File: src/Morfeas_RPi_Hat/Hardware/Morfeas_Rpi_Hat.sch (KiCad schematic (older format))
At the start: 49 parts, among them J1 Power IN, J2 RPi_header, J3 CAN0_Power+, J4 CAN1_Power+, J5 RS_232, Q1 SUM110P06, Q2 SUM110P06, U1 DS3231, U2 TSR2-2450, U3 TLV70433, U4 SP3232, U5 24AA08, U6 MAX9611, U7 MAX9611

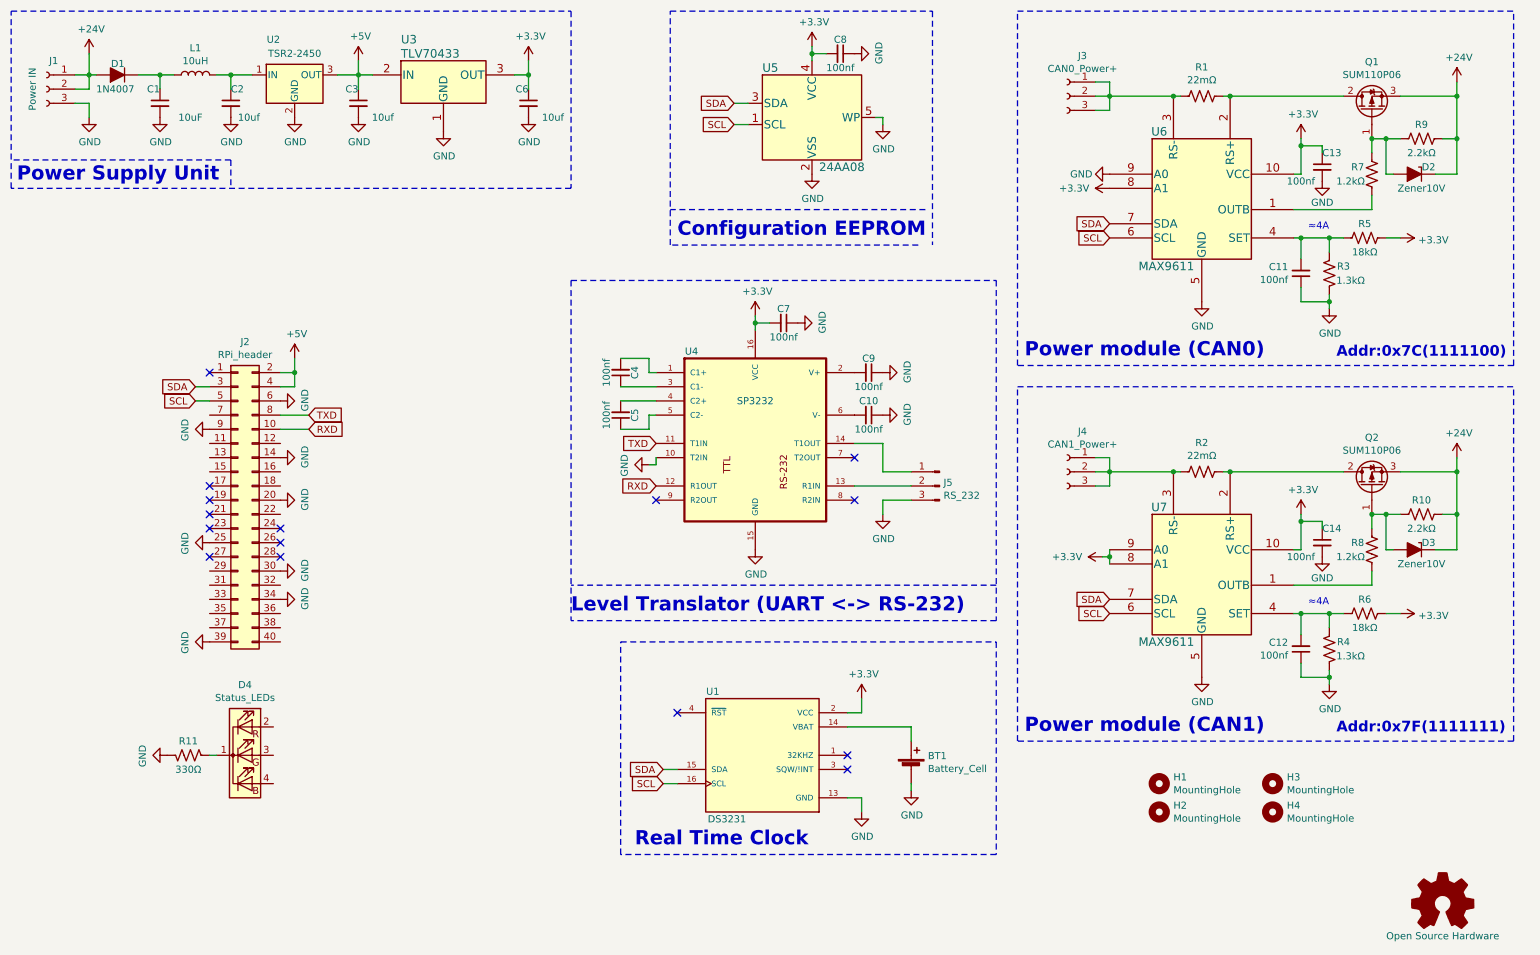
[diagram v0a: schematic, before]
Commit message: Update Morfeas_RPi_hat
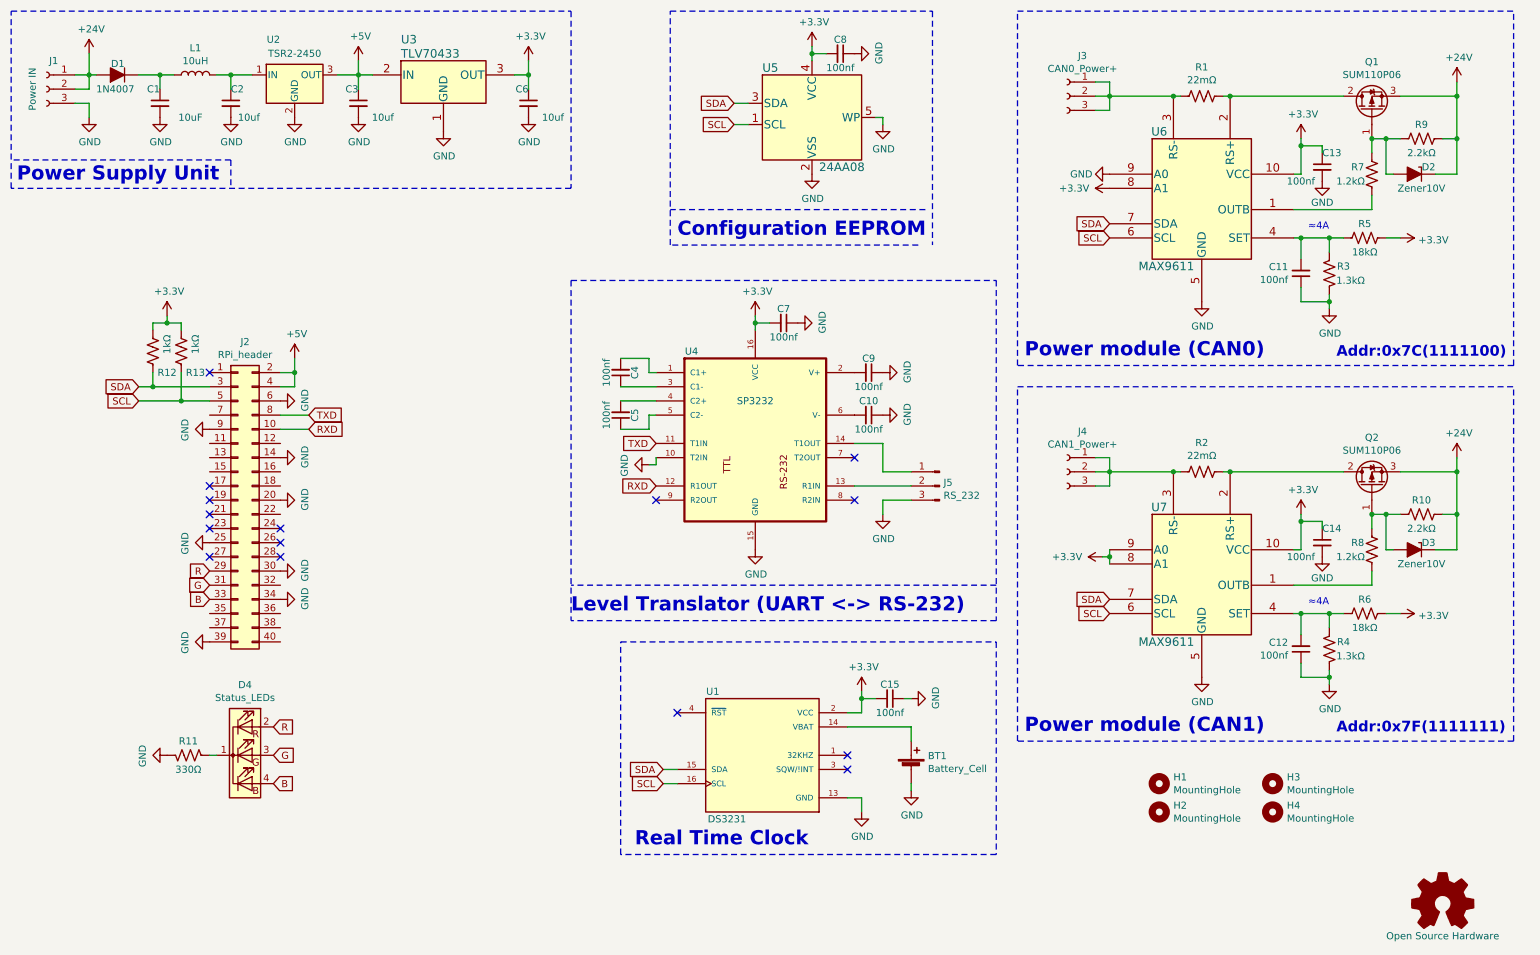
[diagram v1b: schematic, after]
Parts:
- added C15: 100nf, Capacitors_SMD:C_0805, symbol Device:C_Small
- added R12, R13: 1kΩ, Resistors_SMD:R_1206, symbol Device:R_US
- D4: footprint LED_THT:LED_D5.0mm-4_RGB -> Pin_Headers:Pin_Header_Straight_1x04_Pitch2.54mm
- J5: footprint Connector_PinHeader_2.54mm:PinHeader_1x03_P2.54mm_Horizontal -> Pin_Headers:Pin_Header_Straight_1x03_Pitch2.54mm
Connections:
- net +3V3: now also C15.2, R12.1, R13.1
- net GND: now also C15.1
- net SCL: now also R13.2
- net SDA: now also R12.2
- net R: now reaches J2.29 (Pin_29)
- net R: now also D4.2 (RA)
- net G: now reaches J2.31 (Pin_31)
- net G: now also D4.3 (GA)
- net B: now reaches J2.33 (Pin_33)
- net B: now also D4.4 (BA)
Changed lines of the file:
@@
 Wire Wire Line
 	6550 6100 6550 6200
-$Comp
-L power:+3.3V #PWR017
-U 1 1 5E05BB44
-P 6550 5400
-F 0 "#PWR017" H 6550 5250 50  0001 C CNN
-F 1 "+3.3V" H 6565 5573 50  0000 C CNN
-F 2 "" H 6550 5400 50  0001 C CNN
-F 3 "" H 6550 5400 50  0001 C CNN
-	1    6550 5400
-	1    0    0    -1
-$EndComp
 Wire Wire Line
 	6450 5500 6550 5500
@@
 	0    1    1    0
 $EndComp
-Text GLabel 1850 3200 0    50   Input ~ 0
+Text GLabel 1450 3200 0    50   Input ~ 0
 SDA
-Text GLabel 1850 3300 0    50   Input ~ 0
+Text GLabel 1450 3300 0    50   Input ~ 0
 SCL
 Wire Wire Line
-	1850 3200 1950 3200
-Wire Wire Line
-	1850 3300 1950 3300
+	1450 3200 1550 3200
+Wire Wire Line
+	1450 3300 1750 3300
 Text GLabel 2650 3500 2    50   Input ~ 0
 RXD
@@
 F 0 "J5" H 7072 3924 50  0000 R CNN
 F 1 "RS_232" H 7072 3833 50  0000 R CNN
-F 2 "Connector_PinHeader_2.54mm:PinHeader_1x03_P2.54mm_Horizontal" H 7100 3900 50  0001 C CNN
+F 2 "Pin_Headers:Pin_Header_Straight_1x03_Pitch2.54mm" H 7100 3900 50  0001 C CNN
 F 3 "~" H 7100 3900 50  0001 C CNN
 	1    7100 3900
@@
 F 0 "D4" H 2200 6297 50  0000 C CNN
 F 1 "Status_LEDs" H 2200 6206 50  0000 C CNN
-F 2 "LED_THT:LED_D5.0mm-4_RGB" H 2200 5750 50  0001 C CNN
+F 2 "Pin_Headers:Pin_Header_Straight_1x04_Pitch2.54mm" H 2200 5750 50  0001 C CNN
 F 3 "~" H 2200 5750 50  0001 C CNN
 	1    2200 5800
@@
 Text Notes 9700 4750 0    50   ~ 0
 ≈4A
+$Comp
+L Device:C_Small C15
+U 1 1 5E0ACB59
+P 6750 5400
+F 0 "C15" V 6650 5400 50  0000 C CNN
+F 1 "100nf" V 6850 5400 50  0000 C CNN
+F 2 "Capacitors_SMD:C_0805" H 6750 5400 50  0001 C CNN
+F 3 "~" H 6750 5400 50  0001 C CNN
+	1    6750 5400
+	0    1    1    0
+$EndComp
+Wire Wire Line
+	6650 5400 6550 5400
+Connection ~ 6550 5400
+Wire Wire Line
+	6550 5400 6550 5350
+$Comp
+L power:+3.3V #PWR017
+U 1 1 5E05BB44
+P 6550 5350
+F 0 "#PWR017" H 6550 5200 50  0001 C CNN
+F 1 "+3.3V" H 6565 5523 50  0000 C CNN
+F 2 "" H 6550 5350 50  0001 C CNN
+F 3 "" H 6550 5350 50  0001 C CNN
+	1    6550 5350
+	1    0    0    -1
+$EndComp
+$Comp
+L power:GND #PWR045
+U 1 1 5E0C18FA
+P 6900 5400
+F 0 "#PWR045" H 6900 5150 50  0001 C CNN
+F 1 "GND" H 6905 5227 50  0000 C CNN
+F 2 "" H 6900 5400 50  0001 C CNN
+F 3 "" H 6900 5400 50  0001 C CNN
+	1    6900 5400
+	0    -1   -1   0
+$EndComp
+Wire Wire Line
+	6850 5400 6900 5400
+$Comp
+L Device:R_US R12
+U 1 1 5E26B6BA
+P 1550 2950
+F 0 "R12" H 1650 2800 50  0000 C CNN
+F 1 "1kΩ" V 1650 3000 50  0000 C CNN
+F 2 "Resistors_SMD:R_1206" V 1590 2940 50  0001 C CNN
+F 3 "~" H 1550 2950 50  0001 C CNN
+	1    1550 2950
+	1    0    0    -1
+$EndComp
+$Comp
+L Device:R_US R13
+U 1 1 5E27FB7B
+P 1750 2950
+F 0 "R13" H 1850 2800 50  0000 C CNN
+F 1 "1kΩ" V 1850 3000 50  0000 C CNN
+F 2 "Resistors_SMD:R_1206" V 1790 2940 50  0001 C CNN
+F 3 "~" H 1750 2950 50  0001 C CNN
+	1    1750 2950
+	1    0    0    -1
+$EndComp
+$Comp
+L power:+3.3V #PWR046
+U 1 1 5E288B85
+P 1650 2700
+F 0 "#PWR046" H 1650 2550 50  0001 C CNN
+F 1 "+3.3V" H 1665 2873 50  0000 C CNN
+F 2 "" H 1650 2700 50  0001 C CNN
+F 3 "" H 1650 2700 50  0001 C CNN
+	1    1650 2700
+	1    0    0    -1
+$EndComp
+Wire Wire Line
+	1550 2800 1550 2750
+Wire Wire Line
+	1550 2750 1650 2750
+Wire Wire Line
+	1750 2750 1750 2800
+Wire Wire Line
+	1650 2750 1650 2700
+Connection ~ 1650 2750
+Wire Wire Line
+	1650 2750 1750 2750
+Wire Wire Line
+	1550 3100 1550 3200
+Connection ~ 1550 3200
+Wire Wire Line
+	1550 3200 1950 3200
+Wire Wire Line
+	1750 3100 1750 3300
+Connection ~ 1750 3300
+Wire Wire Line
+	1750 3300 1950 3300
+Text GLabel 1950 4500 0    50   Input ~ 0
+R
+Text GLabel 1950 4600 0    50   Input ~ 0
+G
+Text GLabel 1950 4700 0    50   Input ~ 0
+B
+Text GLabel 2400 5600 2    50   Input ~ 0
+R
+Text GLabel 2400 5800 2    50   Input ~ 0
+G
+Text GLabel 2400 6000 2    50   Input ~ 0
+B
 $EndSCHEMATC

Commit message: Update Morfeas_RPi_hat
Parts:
- added Open_Source_hardware1: Open Source Hardware, Symbols:OSHW-Logo2_7.3x6mm_SilkScreen, symbol Graphic:Logo_Open_Hardware_Small
- D1: footprint Diode_THT:D_DO-34_SOD68_P7.62mm_Horizontal -> Diodes_ThroughHole:D_DO-41_SOD81_P10.16mm_Horizontal
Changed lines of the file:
@@
 F 0 "D1" H 1346 921 50  0000 R CNN
 F 1 "1N4007" H 1450 1100 50  0000 R CNN
-F 2 "Diode_THT:D_DO-34_SOD68_P7.62mm_Horizontal" H 1300 1000 50  0001 C CNN
+F 2 "Diodes_ThroughHole:D_DO-41_SOD81_P10.16mm_Horizontal" H 1300 1000 50  0001 C CNN
 F 3 "~" H 1300 1000 50  0001 C CNN
 	1    1300 1000
@@
 Connection ~ 10150 1450
 $Comp
-L Graphic:Logo_Open_Hardware_Small #LOGO1
+L Graphic:Logo_Open_Hardware_Small Open_Source_hardware1
 U 1 1 5E0F6FA7
 P 10650 6850
-F 0 "#LOGO1" H 10650 7125 50  0001 C CNN
+F 0 "Open_Source_hardware1" H 10650 7125 50  0001 C CNN
 F 1 "Open Source Hardware" H 10650 6625 50  0000 C CNN
-F 2 "Symbols:OSHW-Logo2_36.5x30mm_SilkScreen" H 10650 6850 50  0001 C CNN
+F 2 "Symbols:OSHW-Logo2_7.3x6mm_SilkScreen" H 10650 6850 50  0001 C CNN
 F 3 "~" H 10650 6850 50  0001 C CNN
 	1    10650 6850
